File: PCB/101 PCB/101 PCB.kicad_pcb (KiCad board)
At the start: 4 copper layers, 68.6 x 53.3 mm, 52 parts, among them IC101 TPS563202DRLR, IC103 TPS563202DRLR, IC104 DRV8837DSGR, IC105 DRV8837DSGR, J101 TYPE-C-31-M-12, J102 Screw_Terminal_01x02, J103 Screw_Terminal_01x02, J104 Conn_01x04, J105 Conn_01x04, J106 Conn_01x04, J107 Conn_01x04, J108 Conn_01x04, J109 Conn_01x04, J110 Screw_Terminal_01x02, J111 SM04B-SRSS-TB(LF)(SN), U101 ESP32-WROOM-32, U102 STM32G030F6P6, U103 USBLC6-4SC6-ES, U104 LSM6DS3, U106 STM32G431CBUx

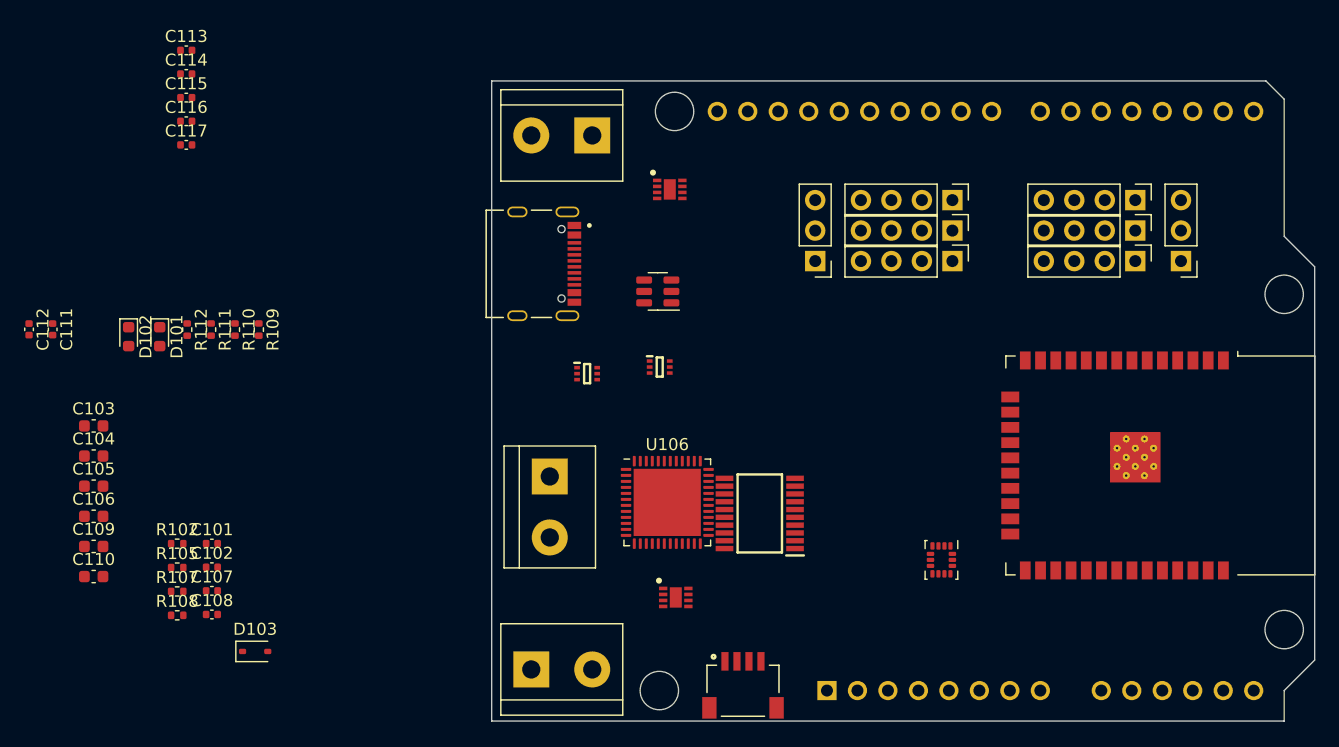
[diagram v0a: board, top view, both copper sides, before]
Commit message: Board layout done
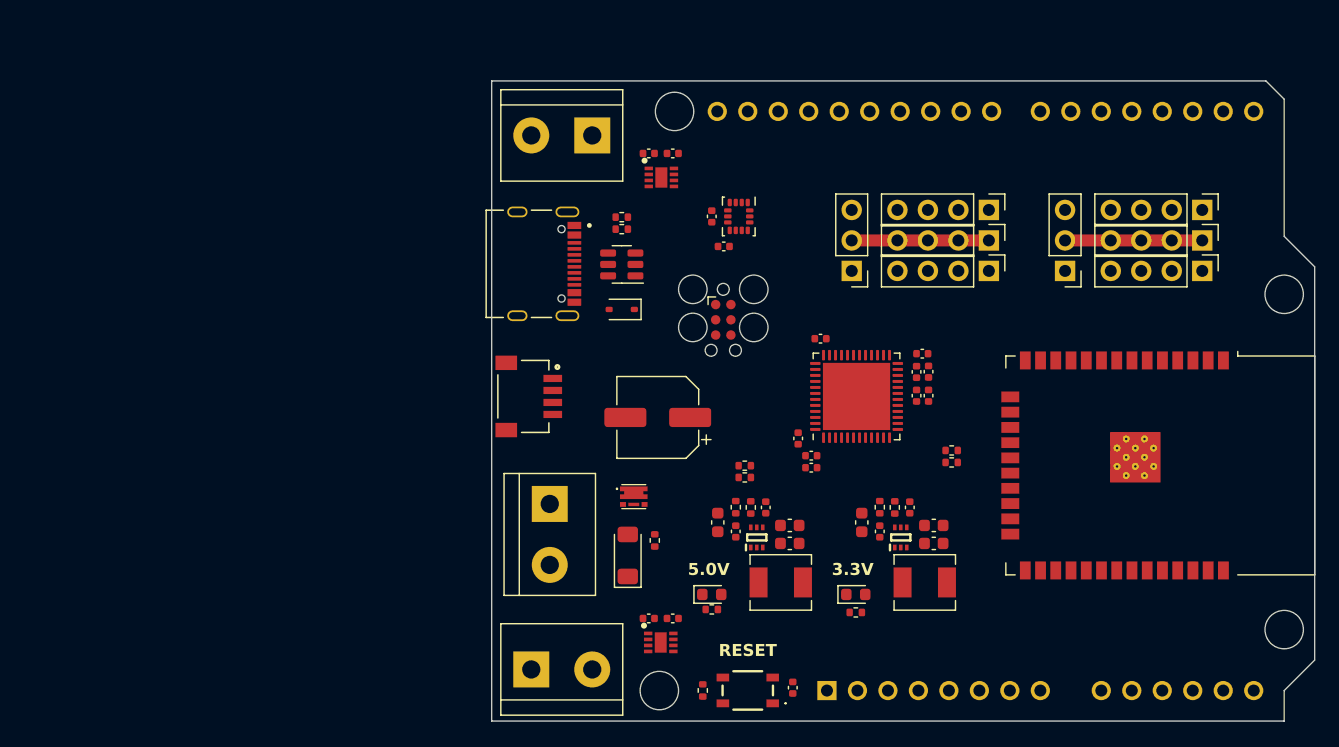
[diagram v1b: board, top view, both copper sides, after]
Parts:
- removed U102: STM32G030F6P6, 101 Footprints:SOP65P640X120-20N
- added C118: 100n, Capacitor_SMD:C_0402_1005Metric, F.Cu at (132.8, 113.0)
- added C119: 47u, Capacitor_SMD:CP_Elec_6.3x5.8, F.Cu at (121.5, 90.5)
- added C120: 100n, Capacitor_SMD:C_0402_1005Metric, F.Cu at (143.5, 85.2)
- added C121: 100n, Capacitor_SMD:C_0402_1005Metric, F.Cu at (134.3, 94.7)
- added C122: 100n, Capacitor_SMD:C_0402_1005Metric, F.Cu at (134.3, 93.7)
- added C123: 100n, Capacitor_SMD:C_0402_1005Metric, F.Cu at (143.1, 86.7)
- added C124: 4u7, Capacitor_SMD:C_0402_1005Metric, F.Cu at (135.1, 83.9)
- added C125: 1u, Capacitor_SMD:C_0402_1005Metric, F.Cu at (144.1, 86.7)
- added C126: 100n, Capacitor_SMD:C_0402_1005Metric, F.Cu at (143.1, 88.7)
- added C127: 1u, Capacitor_SMD:C_0402_1005Metric, F.Cu at (144.1, 88.7)
- added D104: ZMM10V, Diode_SMD:D_MiniMELF, F.Cu at (119.0, 102.0)
- added J112: TC2030, Connector:Tag-Connect_TC2030-IDC-FP_2x03_P1.27mm_Vertical, F.Cu at (127.0, 82.4)
- added L101: 4u7, Inductor_SMD:L_Chilisin_BMRA00040420, F.Cu at (131.8, 104.2)
- added L102: 3u3, Inductor_SMD:L_Chilisin_BMRA00040420, F.Cu at (143.8, 104.2)
- added Q101: DMP3028LFDE, 101 Footprints:DMP2066UFDE7, F.Cu at (119.5, 97.1)
- added R101: 52k, Resistor_SMD:R_0402_1005Metric, F.Cu at (129.2, 98.0)
- added R103: 2k2, Resistor_SMD:R_0402_1005Metric, F.Cu at (126.0, 106.5)
- added R104: 31k, Resistor_SMD:R_0402_1005Metric, F.Cu at (141.2, 98.0)
- added R106: 1k5, Resistor_SMD:R_0402_1005Metric, F.Cu at (138.0, 106.8)
- added R113: 330R, Resistor_SMD:R_0402_1005Metric, F.Cu at (146.0, 93.2)
- added R114: 330R, Resistor_SMD:R_0402_1005Metric, F.Cu at (146.0, 94.2)
- added S101: TS20-42-25-WT-160-SMT-TR, MSL Footprints:TS204225WT160SMTTRMSL, F.Cu at (129.0, 113.2)
- R107: value 5k1 -> 10k
- R108: value 5k1 -> 330R
- R110: value 10k -> 1k
- R112: value 3k3 -> 1k
- moved C110 70.1 mm to (144.5, 101.0), turned to 180 degrees
- moved C109 70.0 mm to (144.5, 99.5), turned to 180 degrees
- moved D102 64.3 mm to (138.0, 105.2), turned to 0 degrees
- moved C106 64.0 mm to (138.5, 99.2), turned to 90 degrees
- moved C113 62.3 mm to (122.8, 107.2), turned to 180 degrees
- moved C114 59.5 mm to (120.8, 107.2)
- moved C108 58.8 mm to (142.5, 98.0), turned to 90 degrees
- moved R105 58.8 mm to (140.0, 98.0), turned to -90 degrees
- moved C103 58.6 mm to (132.5, 99.5), turned to 180 degrees
- moved C104 58.5 mm to (132.5, 101.0), turned to 180 degrees
- moved C112 57.7 mm to (126.0, 73.8)
- moved C117 56.6 mm to (133.2, 92.2), turned to -90 degrees
- moved C111 56.3 mm to (127.0, 76.2), turned to 180 degrees
- moved C107 55.9 mm to (140.0, 100.0), turned to 90 degrees
- moved C105 52.1 mm to (126.5, 99.2), turned to 90 degrees
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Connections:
- A101 pad 10: unconnected-(A101-A1-Pad10) -> GPIO26
- A101 pad 11: unconnected-(A101-A2-Pad11) -> GPIO27
- A101 pad 12: unconnected-(A101-A3-Pad12) -> GPIO32
- A101 pad 13: unconnected-(A101-SDA/A4-Pad13) -> GPIO33
- A101 pad 14: unconnected-(A101-SCL/A5-Pad14) -> GPIO15
- A101 pad 17: unconnected-(A101-D2-Pad17) -> IO0
- A101 pad 18: unconnected-(A101-D3-Pad18) -> GPIO2
- A101 pad 19: unconnected-(A101-D4-Pad19) -> GPIO4
- A101 pad 20: unconnected-(A101-D5-Pad20) -> GPIO12
- A101 pad 21: unconnected-(A101-D6-Pad21) -> GPIO13
- A101 pad 22: unconnected-(A101-D7-Pad22) -> GPIO14
- A101 pad 23: unconnected-(A101-D8-Pad23) -> GPIO17
- A101 pad 24: unconnected-(A101-D9-Pad24) -> GPIO16
- A101 pad 9: unconnected-(A101-A0-Pad9) -> GPIO25
- J101 pad A5: /CC1 -> CC1
- J101 pad B5: /CC2 -> CC2
- J110 pad 1: +BATT -> VIN
- R107 pad 1: /CC1 -> EN
- R107 pad 2: GND -> +3V3
- R108 pad 1: /CC2 -> /RP_PMOS_G
- R109 pad 2: VBUS/2 -> VBUS/11
- R110 pad 1: VBUS/2 -> VBUS/11
- R111 pad 2: BATT/4 -> BATT/11
- R112 pad 1: BATT/4 -> BATT/11
- U101 pad 4: BATT/4 -> BATT/11
- U101 pad 5: VBUS/2 -> VBUS/11
- U103 pad 1: /CC1 -> CC2
- U103 pad 3: /CC2 -> CC1
- U103 pad 4: USB_DP -> USB_DN
- U103 pad 6: USB_DN -> USB_DP
- U106 pad 1: unconnected-(U106-VBAT-Pad1) -> +3.3V
- U106 pad 10: unconnected-(U106-PA2-Pad10) -> ESP32_RX
- U106 pad 11: unconnected-(U106-PA3-Pad11) -> ESP32_TX
- U106 pad 14: unconnected-(U106-PA6-Pad14) -> S4
- U106 pad 15: unconnected-(U106-PA7-Pad15) -> S5
- U106 pad 17: unconnected-(U106-PB0-Pad17) -> S6
- U106 pad 18: unconnected-(U106-PB1-Pad18) -> S7
- U106 pad 2: unconnected-(U106-PC13-Pad2) -> M2_IN2
- U106 pad 20: unconnected-(U106-VREF+-Pad20) -> VREF+
- U106 pad 21: unconnected-(U106-VDDA-Pad21) -> +3.3V
- U106 pad 22: unconnected-(U106-PB10-Pad22) -> S2
- U106 pad 23: unconnected-(U106-VDD-Pad23) -> +3.3V
- U106 pad 24: unconnected-(U106-PB11-Pad24) -> S3
- U106 pad 28: unconnected-(U106-PB15-Pad28) -> VBUS/11
- U106 pad 29: unconnected-(U106-PC6-Pad29) -> M1_IN1
- U106 pad 33: unconnected-(U106-PA11-Pad33) -> USB_DN
- U106 pad 34: unconnected-(U106-PA12-Pad34) -> USB_DP
- U106 pad 35: unconnected-(U106-VDD-Pad35) -> +3.3V
- U106 pad 36: unconnected-(U106-PA13-Pad36) -> SWDIO
- U106 pad 37: unconnected-(U106-PA14-Pad37) -> SWCLK
- U106 pad 38: unconnected-(U106-PA15-Pad38) -> SCL
- U106 pad 41: unconnected-(U106-PB3-Pad41) -> SWO
- U106 pad 42: unconnected-(U106-PB4-Pad42) -> CC2
- U106 pad 44: unconnected-(U106-PB6-Pad44) -> CC1
- U106 pad 45: unconnected-(U106-PB7-Pad45) -> SDA
- U106 pad 46: unconnected-(U106-PB8-Pad46) -> M1_IN2
- U106 pad 47: unconnected-(U106-PB9-Pad47) -> M2_IN1
- U106 pad 48: unconnected-(U106-VDD-Pad48) -> +3.3V
- U106 pad 49: unconnected-(U106-VSS-Pad49) -> GND
- U106 pad 5: unconnected-(U106-PF0-Pad5) -> BATT/11
- U106 pad 7: unconnected-(U106-PG10-Pad7) -> NRST
- U106 pad 8: unconnected-(U106-PA0-Pad8) -> S0
- U106 pad 9: unconnected-(U106-PA1-Pad9) -> S1
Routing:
- net VDDIO2: track 0.00 -> 11.4 mm
- net VDDIO1: track 0.00 -> 11.4 mm
- added copper zone on In1.Cu, net GND
- added copper zone on In2.Cu, net GND
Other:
- board text added: "3.3V"
- board text added: "5.0V"
- board text added: "RESET"

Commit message: Firmware working
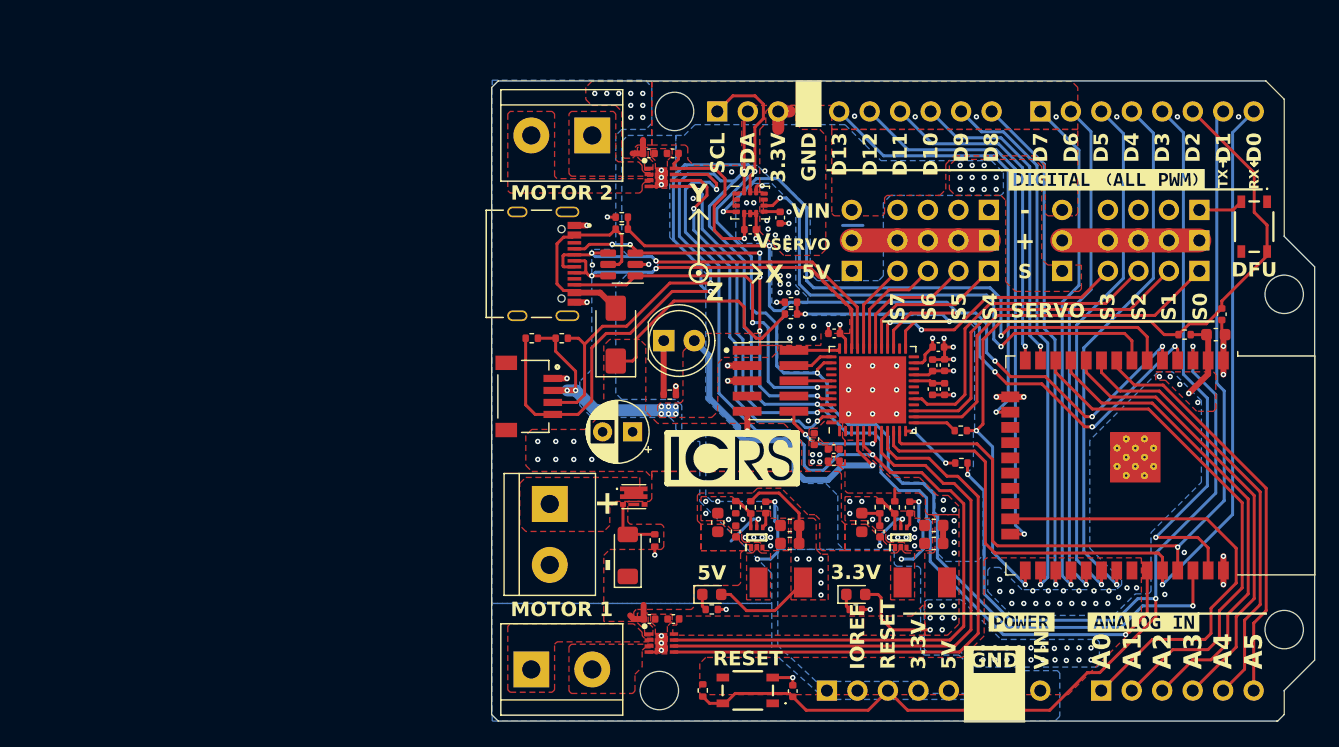
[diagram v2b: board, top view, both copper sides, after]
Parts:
- removed D103: BAT760-115, Diode_SMD:D_SOD-323
- removed the G*** at (141.5, 89.0)
- removed J112: TC2030, Connector:Tag-Connect_TC2030-IDC-FP_2x03_P1.27mm_Vertical
- removed R113: 330R, Resistor_SMD:R_0402_1005Metric
- added C1: 100n, Capacitor_SMD:C_0402_1005Metric, F.Cu at (168.5, 81.9)
- added C2: 22u, Capacitor_SMD:C_0603_1608Metric, F.Cu at (168.0, 83.6)
- added D1: LED_R, LED_THT:LED_D5.0mm, F.Cu at (122.0, 84.1)
- added D2: SK34, 101 Footprints:SK34, F.Cu at (118.0, 83.6)
- added G***: LOGO, 101 Footprints:ICRS_text_neg_4mm, F.Cu at (127.7, 93.8)
- added G***: LOGO, 101 Footprints:Digital 1.4mm, F.Cu at (158.9, 70.7)
- added G***: LOGO, 101 Footprints:power analog in 1.6mm, F.Cu at (157.8, 107.5)
- added G***: LOGO, 101 Footprints:ICRS Medium, B.Cu at (129.5, 91.4)
- added G***: LOGO, 101 Footprints:DC_logo_4mm, B.Cu at (114.7, 107.7)
- added J1: Conn_01x10, 101 Footprints:PinHeader_1x10_P2.54mm_Vertical, F.Cu at (126.5, 65.0)
- added J2: Conn_ARM_JTAG_SWD_10, Connector_PinHeader_1.27mm:PinHeader_2x05_P1.27mm_Vertical_SMD, F.Cu at (130.9, 87.4)
- added J3: Conn_01x08, 101 Footprints:PinHeader_1x08_P2.54mm_Vertical, F.Cu at (153.4, 65.0)
- added J4: Conn_01x08, 101 Footprints:PinHeader_1x08_P2.54mm_Vertical, F.Cu at (135.6, 113.3)
- added J5: Conn_01x06, 101 Footprints:PinHeader_1x06_P2.54mm_Vertical, F.Cu at (158.5, 113.3)
- added R1: 10k, Resistor_SMD:R_0402_1005Metric, F.Cu at (165.4, 83.6)
- added R2: 330R, Resistor_SMD:R_0402_1005Metric, F.Cu at (146.8, 91.6)
- added R3: 330R, Resistor_SMD:R_0402_1005Metric, F.Cu at (122.5, 88.6)
- added R4: 2k2, Resistor_SMD:R_0402_1005Metric, F.Cu at (113.5, 83.9)
- added R5: 2k2, Resistor_SMD:R_0402_1005Metric, F.Cu at (111.0, 83.9)
- added REF**: KiCad-Logo2_5mm_SilkScreen, Symbol:KiCad-Logo2_5mm_SilkScreen, B.Cu at (149.9, 108.0)
- added REF**: WEEE-Logo_4.2x6mm_SilkScreen, Symbol:WEEE-Logo_4.2x6mm_SilkScreen, B.Cu at (160.0, 108.0)
- added REF**: ESD-Logo_6.6x6mm_SilkScreen, Symbol:ESD-Logo_6.6x6mm_SilkScreen, B.Cu at (167.6, 108.0)
- added S102: TS20-42-25-WT-160-SMT-TR, MSL Footprints:TS204225WT160SMTTRMSL, F.Cu at (171.2, 74.6)
- A101: footprint 101 Footprints:ICRS_101_UNO_R3 -> 101 Footprints:ICRS_101_UNO_R3_NO_PINS
- C119: footprint Capacitor_SMD:CP_Elec_6.3x5.8 -> Capacitor_THT:CP_Radial_D5.0mm_P2.50mm
- J101: footprint 101 Footprints:HRO_TYPE-C-31-M-12 -> MSL Footprints:HRO_TYPE-C-31-M-12
- J102, J103, J110: footprint TerminalBlock:TerminalBlock_bornier-2_P5.08mm -> 101 Footprints:TerminalBlock_bornier-2_P5.08mm
- J104, J105, J106, J107, J108, J109: footprint Connector_PinHeader_2.54mm:PinHeader_1x04_P2.54mm_Vertical -> 101 Footprints:PinHeader_1x04_P2.54mm_Vertical
- JP101, JP102: footprint Connector_PinHeader_2.54mm:PinHeader_1x03_P2.54mm_Vertical -> 101 Footprints:PinHeader_1x03_P2.54mm_Vertical
- L101, L102: footprint Inductor_SMD:L_Chilisin_BMRA00040420 -> 101 Footprints:L_Chilisin_BMRA00040415
- R101: value 52k -> 27k
- R102, R105: value 10k -> 5k1
- R103: value 2k2 -> 1k2
- R104: value 31k -> 16k
- R106: value 1k5 -> 330R
- U101: footprint RF_Module:ESP32-WROOM-32 -> 101 Footprints:ESP32-WROOM-32
- moved R111 14.2 mm to (132.6, 81.9)
- moved R112 14.2 mm to (132.6, 80.9)
- moved C111 5.28 mm to (131.7, 73.8), turned to -90 degrees
- moved C112 3.38 mm to (129.2, 74.8), turned to 0 degrees
- moved C119 2.41 mm to (119.4, 91.7)
- moved C121 1.95 mm to (136.2, 94.1)
- moved C122 1.95 mm to (136.2, 93.1)
- moved U104 1.49 mm to (129.2, 72.6), turned to 0 degrees
- moved C120 1.45 mm to (144.9, 84.6)
- moved C123 1.45 mm to (144.4, 86.2)
- moved C125 1.45 mm to (145.4, 86.1)
- moved C126 1.45 mm to (144.4, 88.1)
- moved C127 1.45 mm to (145.4, 88.1)
- moved U106 1.45 mm to (139.4, 88.2)
- moved C117 1.34 mm to (134.5, 92.3)
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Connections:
- C102 pad 1: +BATT -> VIN
- C105 pad 1: +BATT -> VIN
- C106 pad 1: +5V -> VIN
- C107 pad 1: +5V -> VIN
- C114 pad 1: +BATT -> VIN
- C116 pad 1: +BATT -> VIN
- C119 pad 1: +BATT -> VIN
- D104 pad 1: +BATT -> VIN
- IC101 pad 1: +BATT -> VIN
- IC101 pad 5: +BATT -> VIN
- IC103 pad 1: +5V -> VIN
- IC103 pad 5: +5V -> VIN
- IC104 pad 1: +BATT -> VIN
- IC105 pad 1: +BATT -> VIN
- J101 pad S2: unconnected-(J101-SHIELD-PadS1) -> unconnected-(J101-SHIELD-PadS2)
- J101 pad S3: unconnected-(J101-SHIELD-PadS1) -> unconnected-(J101-SHIELD-PadS3)
- J101 pad S4: unconnected-(J101-SHIELD-PadS1) -> unconnected-(J101-SHIELD-PadS4)
- J110 pad 1: VIN -> +BATT
- J111 pad 2: +3V3 -> +3.3V
- JP101 pad 1: +3V3 -> +5V
- JP101 pad 3: +5V -> VIN
- JP102 pad 1: +3V3 -> +5V
- JP102 pad 3: +5V -> VIN
- Q101 pad 1: VIN -> +BATT
- Q101 pad 2: VIN -> +BATT
- Q101 pad 4: +BATT -> VIN
- Q101 pad 5: VIN -> +BATT
- Q101 pad 6: VIN -> +BATT
- Q101 pad 7: +BATT -> VIN
- Q101 pad 8: (no net) -> +BATT
- R107 pad 2: +3V3 -> +3.3V
- R111 pad 1: +BATT -> VIN
- R111 pad 2: BATT/11 -> VIN/11
- R112 pad 1: BATT/11 -> VIN/11
- R114 pad 1: unconnected-(R114-Pad1) -> /STM32_EN
- U101 pad 4: BATT/11 -> VIN/11
- U106 pad 12: unconnected-(U106-PA4-Pad12) -> /STM32_EN
- U106 pad 13: unconnected-(U106-PA5-Pad13) -> /STM32_IO0
- U106 pad 14: S4 -> S0
- U106 pad 15: S5 -> S1
- U106 pad 17: S6 -> S2
- U106 pad 18: S7 -> unconnected-(U106-PB1-Pad18)
- U106 pad 2: M2_IN2 -> unconnected-(U106-PC13-Pad2)
- U106 pad 22: S2 -> unconnected-(U106-PB10-Pad22)
- U106 pad 24: S3 -> unconnected-(U106-PB11-Pad24)
- U106 pad 25: unconnected-(U106-PB12-Pad25) -> VIN/11
- U106 pad 27: unconnected-(U106-PB14-Pad27) -> VBUS/11
- U106 pad 28: VBUS/11 -> S3
- U106 pad 29: M1_IN1 -> S4
- U106 pad 30: unconnected-(U106-PA8-Pad30) -> S5
- U106 pad 31: unconnected-(U106-PA9-Pad31) -> S6
- U106 pad 32: unconnected-(U106-PA10-Pad32) -> S7
- U106 pad 4: unconnected-(U106-PC15-Pad4) -> /STM_LED_A
- U106 pad 46: M1_IN2 -> M2_IN2
- U106 pad 5: BATT/11 -> MOTOR_SLEEP
- U106 pad 8: S0 -> M1_IN1
- U106 pad 9: S1 -> M1_IN2
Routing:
- net SCL: track 0.00 -> 133.7 mm, vias 0 -> 4
- net SDA: track 0.00 -> 116.2 mm, vias 0 -> 4
- net EN: track 0.00 -> 97.6 mm, vias 0 -> 3
- net MOTOR_SLEEP: track 0.00 -> 89.0 mm, vias 0 -> 2
- net ESP32_RX: track 0.00 -> 76.3 mm, vias 0 -> 1
- net ESP32_TX: track 0.00 -> 72.0 mm, vias 0 -> 1
- net +3.3V: track 0.00 -> 69.4 mm, vias 0 -> 76
- net VBUS/11: track 0.00 -> 68.0 mm, vias 0 -> 5
- net IO0: track 0.00 -> 66.7 mm, vias 0 -> 2
- net IMU_INT1: track 0.00 -> 50.9 mm, vias 0 -> 2
- net M1_IN2: track 0.00 -> 48.1 mm
- net VIN/11: track 0.00 -> 47.3 mm, vias 0 -> 5
- net M1_IN1: track 0.00 -> 47.0 mm
- net GPIO2: track 0.00 -> 46.0 mm, vias 0 -> 1
- net GPIO23: track 0.00 -> 45.4 mm, vias 0 -> 1
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- added copper zone on B.Cu, net +3.3V
- added copper zone on F.Cu, net +3.3V
- added copper zone on B.Cu, net +5V
- added copper zone on F.Cu, net +5V
- added copper zone on F.Cu, net +BATT
- added copper zone on F.Cu, net /3V3_SW
- added copper zone on F.Cu, net /5V_SW
- added copper zone on F.Cu, net /M1_OUT1
- added copper zone on F.Cu, net /M1_OUT2
- added copper zone on F.Cu, net /M2_OUT1
- added copper zone on F.Cu, net /M2_OUT2
- added copper zone on F.Cu, net GND
- added copper zone on B.Cu, net VIN
- added copper zone on F.Cu, net VIN
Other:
- outline, holes or cut-outs redrawn
- board text added: "+"
- board text added: "-"
- board text added: "1"
- board text added: "101"
- board text added: "2"
- board text added: "5V"
- board text added: "A0"
- board text added: "A1"
- board text added: "A2"
- board text added: "A3"
- board text added: "A4"
- board text added: "A5"
- board text added: "D0"
- board text added: "D1"
- board text added: "D10"
- board text added: "D11"
- board text added: "D12"
- board text added: "D13"
- board text added: "D2"
- board text added: "D3"
- board text added: "D4"
- board text added: "D5"
- board text added: "D6"
- board text added: "D7"
- board text added: "D8"
- board text added: "D9"
- board text added: "DEVKIT"
- board text added: "DFU"
- board text added: "Designed by Ben Smith 2023"
- board text added: "GND"
- board text added: "IOREF"
- board text added: "Input: 5-11V 2A"
- board text added: "MOTOR 1"
- board text added: "MOTOR 2"
- board text added: "RX"
- board text added: "S"
- board text added: "S0"
- board text added: "S1"
- board text added: "S2"
- board text added: "S3"
- board text added: "S4"
- board text added: "S5"
- board text added: "S6"
- board text added: "S7"
- board text added: "SCL"
- board text added: "SDA"
- board text added: "SERVO"
- board text added: "Select servo voltage with jumper"
- board text added: "TX"
- board text added: "This belongs to:"
- board text added: "V1.0"
- board text added: "VIN"
- board text added: "V_{SERVO}"
- board text added: "X"
- board text added: "Y"
- board text added: "Z"
- board text removed: "5.0V"
